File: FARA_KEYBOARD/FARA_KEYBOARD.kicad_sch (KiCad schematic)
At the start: 32 parts, among them J1 Conn_01x07_Pin, J10 Conn_01x02, J11 Screw_Terminal_01x02, J12 Screw_Terminal_01x02, J13 Conn_01x02, J2 Conn_01x20, J3 Conn_01x20, J4 Conn_01x04, J5 Conn_01x03, J6 Conn_01x03, J7 Conn_01x03, J8 Conn_01x03, J9 Conn_01x03, Q1 AO3400A, Q2 AO3400A, Q3 AO3400A, SW1 SW_Push, SW2 SW_Push, SW3 SW_Push, SW4 SW_Push, SW5 SW_Push, SW6 SW_Push, U1 Raspberri_Pi_Pico

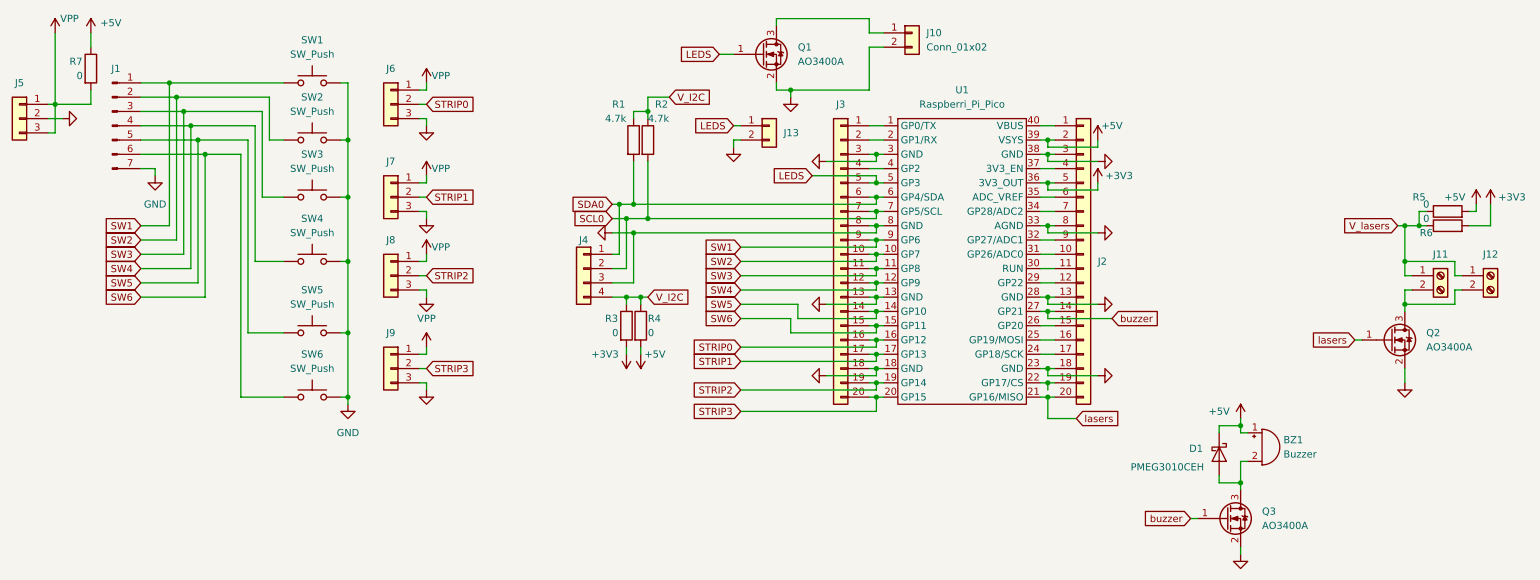
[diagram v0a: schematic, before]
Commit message: v0.7 form was corrected
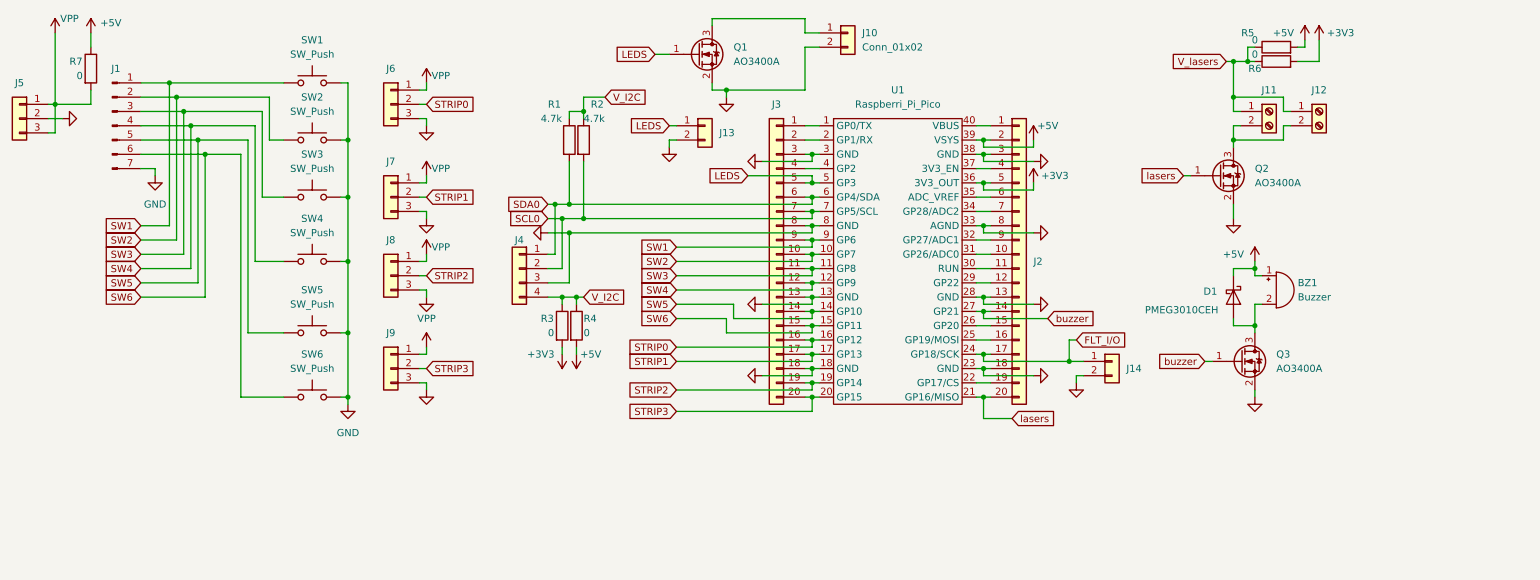
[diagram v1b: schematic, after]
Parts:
- added J14: Conn_01x02, Connector_PinSocket_2.54mm:PinSocket_1x02_P2.54mm_Vertical, symbol Connector_Generic:Conn_01x02
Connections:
- net GND: now also J14.2 (Pin_2)
- net FLT_I/O: now reaches J2.17 (Pin_17), U1.24 (GP18/SCK)
- net FLT_I/O: now also J14.1 (Pin_1)
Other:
- moved on the sheet: BZ1, D1, J10, J11, J12, J13, J2, J3, J4, Q1, Q2, Q3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
